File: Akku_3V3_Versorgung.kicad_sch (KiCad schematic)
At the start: 29 parts, among them J1 USB_5V_IN, J2 OUT_3V3, Q1 FS8205A, U1 TP4056, U2 DW01A, U3 MT3608, U4 AP2112K-3.3

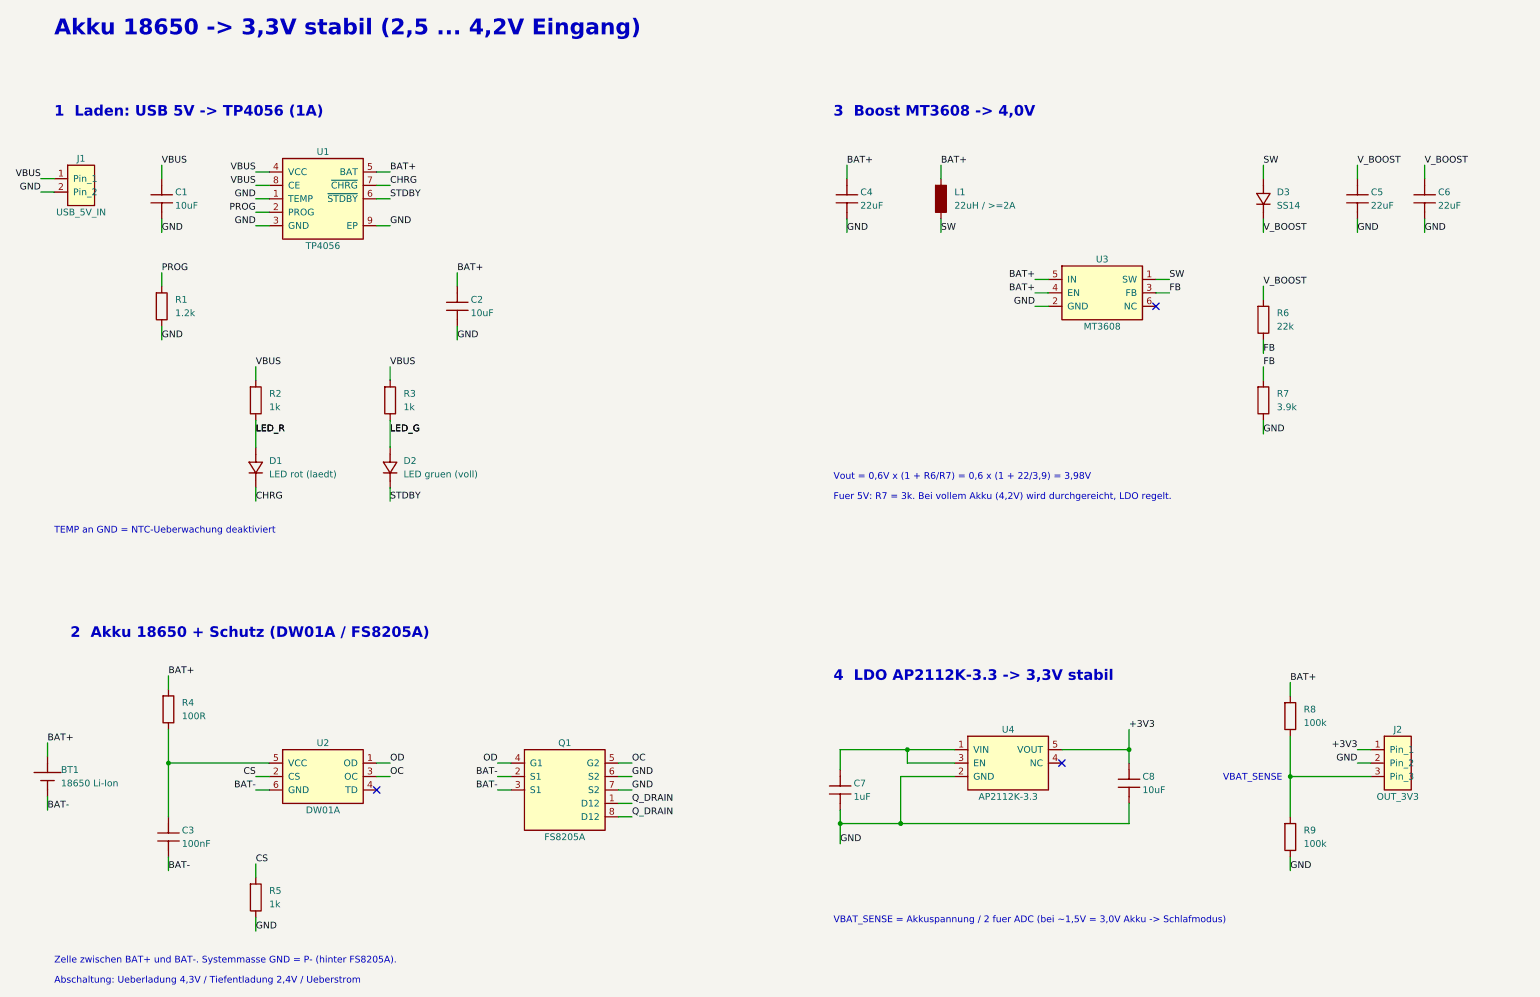
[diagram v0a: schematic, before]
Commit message: docu
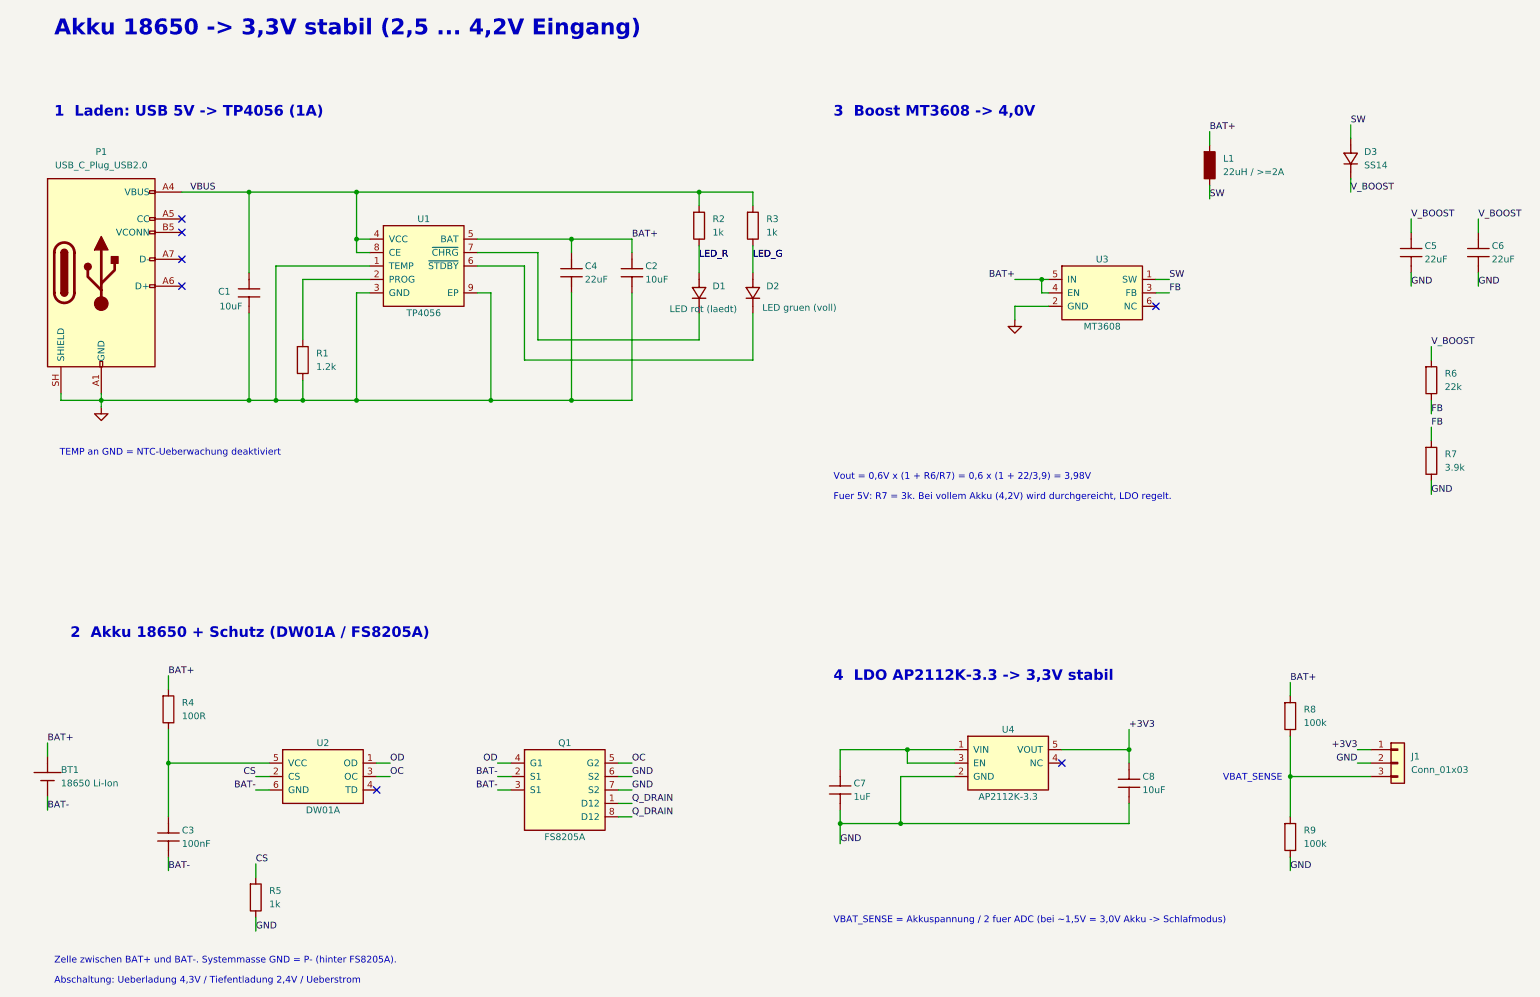
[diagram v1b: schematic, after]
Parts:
- removed J1: USB_5V_IN, Connector_JST:JST_PH_B2B-PH-K_1x02_P2.00mm_Vertical, symbol Akku3V3:Conn_01x02
- removed J2: OUT_3V3, Connector_JST:JST_PH_B2B-PH-K_1x03_P2.00mm_Vertical, symbol Akku3V3:Conn_01x03
- added J1: Conn_01x03, Connector_JST:JST_EH_B3B-EH-A_1x03_P2.50mm_Vertical, symbol Connector_Generic:Conn_01x03
- added P1: USB_C_Plug_USB2.0, Connector_USB:USB_C_Receptacle_GCT_USB4105-xx-A_16P_TopMnt_Horizontal, symbol Connector:USB_C_Plug_USB2.0
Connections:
- net +3V3: now also J1.1 (Pin_1)
- net GND: now also J1.2 (Pin_2), P1.A1 (GND), P1.A12 (GND), P1.B1 (GND), P1.B12 (GND), P1.SH (SHIELD)
- net VBUS: now also P1.A4 (VBUS), P1.A9 (VBUS), P1.B4 (VBUS), P1.B9 (VBUS)
- net at R8.2, R9.1: now also J1.3 (Pin_3)
- net CHRG: no longer names the net of D1.1 (K), U1.7 (~{CHRG})
- net PROG: no longer names the net of R1.1, U1.2 (PROG)
- net STDBY: no longer names the net of D2.1 (K), U1.6 (~{STDBY})
- no-connect marks 3 -> 7
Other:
- moved on the sheet: C1, C2, C4, C5, C6, D1, D2, D3, L1, R1, R2, R3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
